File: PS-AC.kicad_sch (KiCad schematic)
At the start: 19 parts, among them J1 Conn_01x02, J2 Conn_01x02, J3 Conn_01x04, Q1 NTZD3154NT1G, U1 HLK-10M05, U2 INA219AxD, U3 AMS1117-3.3

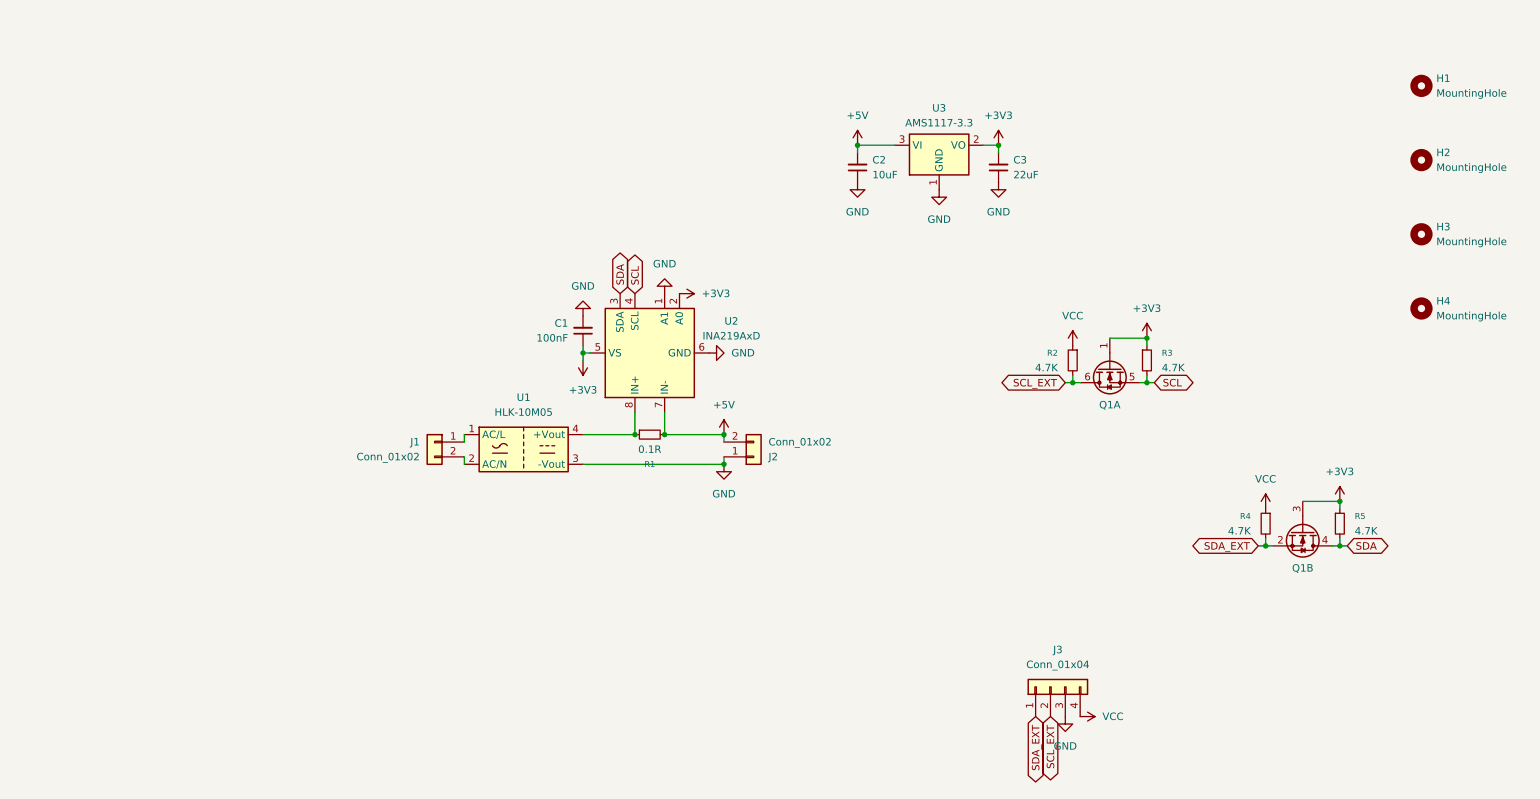
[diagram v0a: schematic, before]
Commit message: update
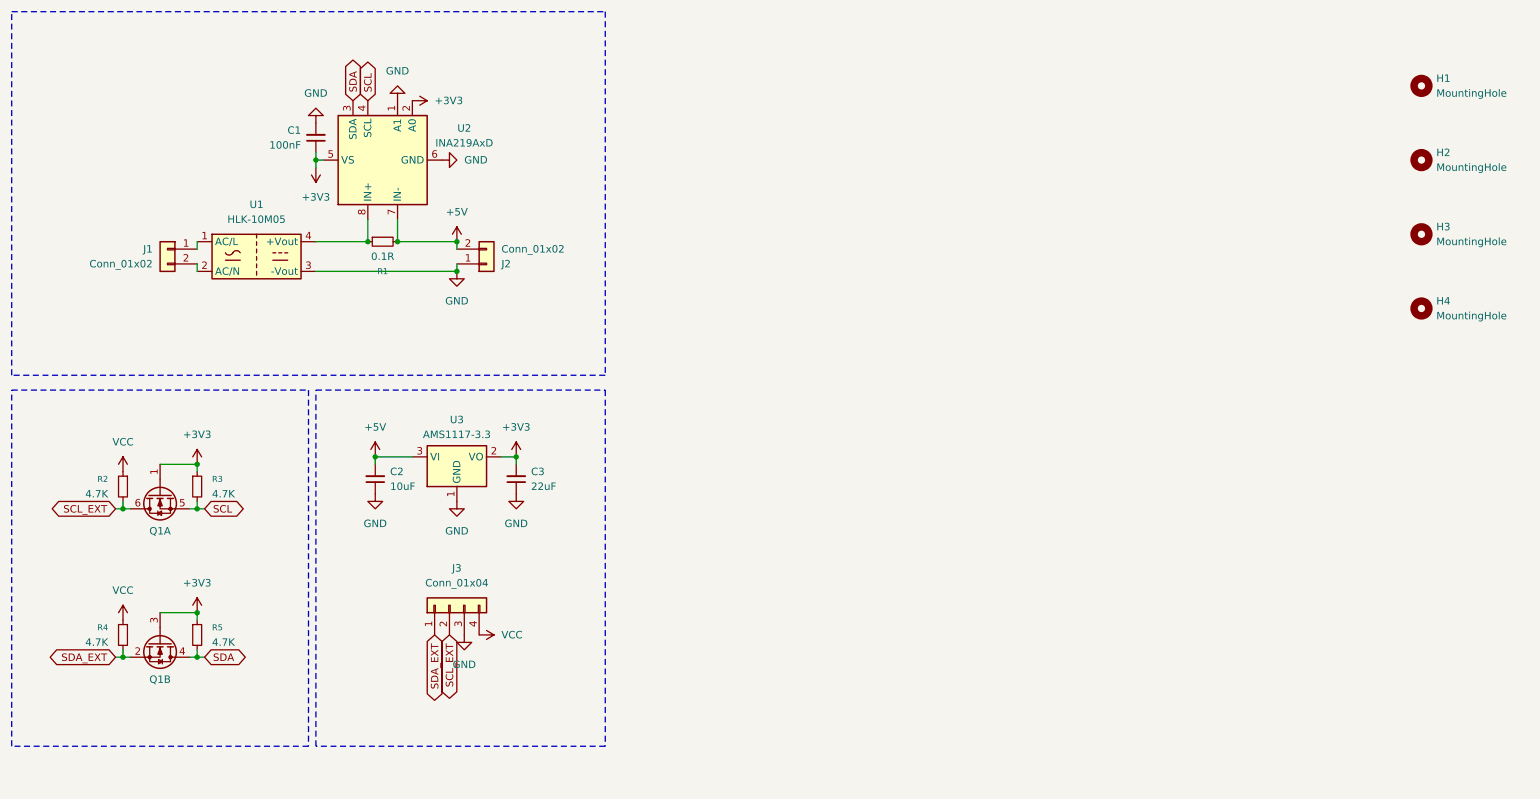
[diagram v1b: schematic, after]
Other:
- company: (none) -> PT. Ruang Industri Indonesia
- title: (none) -> RX-PSU
- moved on the sheet: C1, C2, C3, J1, J2, J3, Q1A, Q1B, R1, R2, R3, R4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
